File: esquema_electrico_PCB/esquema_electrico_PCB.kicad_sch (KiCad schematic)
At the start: 0 parts

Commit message: Aqui la etapa de alimentacion ya está totalmente terminada en el esquematico
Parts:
- added C1, C2, C4: 100nF, Capacitor_THT:C_Disc_D5.0mm_W2.5mm_P5.00mm, symbol PCM_Nuova-Elettronica-Capacitors:Capacitor
- added C3: 22nF, Capacitor_THT:C_Disc_D5.0mm_W2.5mm_P5.00mm, symbol PCM_Nuova-Elettronica-Capacitors:Capacitor
- added F1: Fuse, Fuse:Fuseholder_Cylinder-5x20mm_Schurter_0031_8201_Horizontal_Open, symbol Device:Fuse
- added J1: Barrel_Jack_PTH, Connector_BarrelJack:BarrelJack_GCT_DCJ200-10-A_Horizontal, symbol PCM_SparkFun-Connector:Barrel_Jack_PTH
- added SW1: Switch, PCM_fab:PinHeader_01x02_P2.54mm_Vertical_THT_D1mm, symbol Switch:SW_SPST
- added U1: LM7805MP, Package_TO_SOT_SMD:SOT-223, symbol PCM_Voltage_Regulator_AKL:LM7805MP
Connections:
- new net: J1.1 (PWR), SW1.1 (A)
- new net: F1.1, SW1.2 (B)
- new net +12V: C1.2, C2.2, C3.2, F1.2, U1.1 (IN)
- new net 5V: C4.2, U1.3 (OUT)
- new net GNDREF: C1.1, C2.1, C3.1, C4.1, J1.2 (GND), U1.2
- no-connect marks 0 -> 1
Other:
- note added: "ALIMENTACION"
- title: (none) -> ESQUEMA ELECTRICO

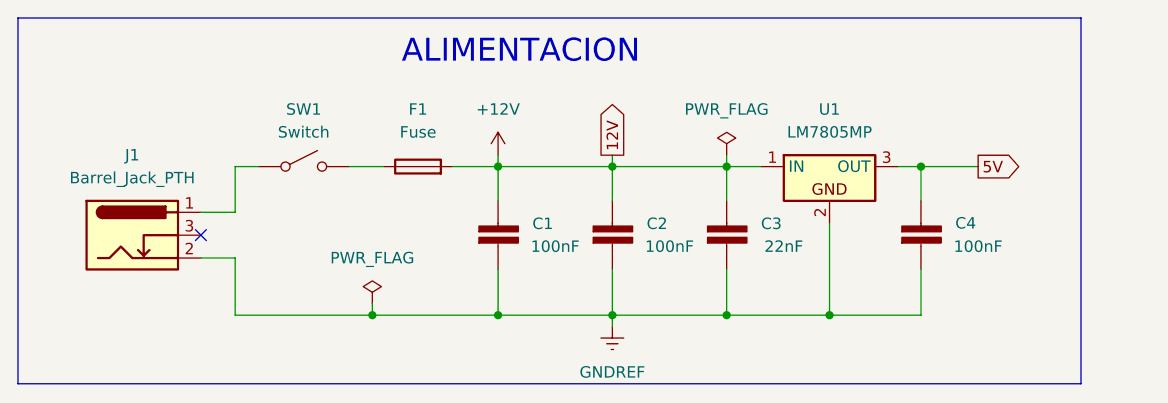
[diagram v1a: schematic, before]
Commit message: Aquí ya está terminada la etapa de alimentación en su totalidad
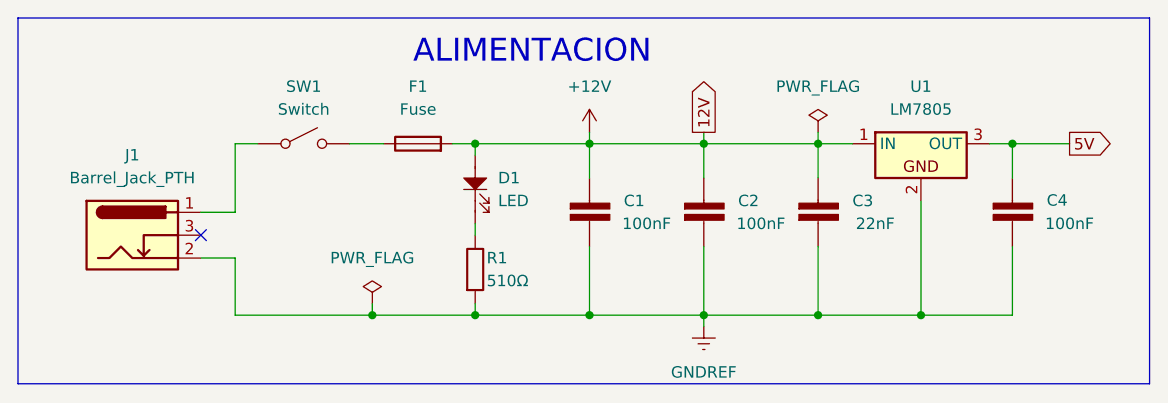
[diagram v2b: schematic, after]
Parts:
- added D1: LED, PCM_SparkFun-LED:LED_5mm_PTH_Red_Silk, symbol PCM_SL_Devices:LED
- added R1: 510Ω, Resistor_THT:R_Axial_DIN0207_L6.3mm_D2.5mm_P7.62mm_Horizontal, symbol PCM_SL_Resistors:Resistor
- U1: value LM7805MP -> LM7805
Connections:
- net +12V: now also D1.2
- net GNDREF: now also R1.1
- new net: D1.1, R1.2
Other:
- moved on the sheet: C1, C2, C3, C4, F1, SW1, U1
